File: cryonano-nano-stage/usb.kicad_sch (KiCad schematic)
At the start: 5 parts, among them J4 10118194-0001LF, U10 ECMF02-2AMX6

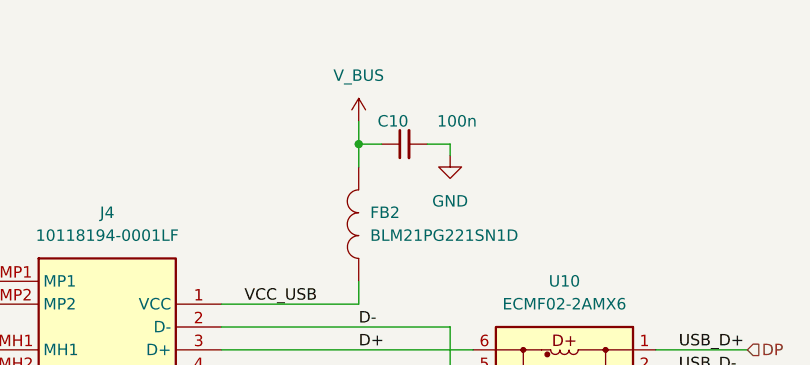
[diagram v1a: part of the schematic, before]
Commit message: partially populated
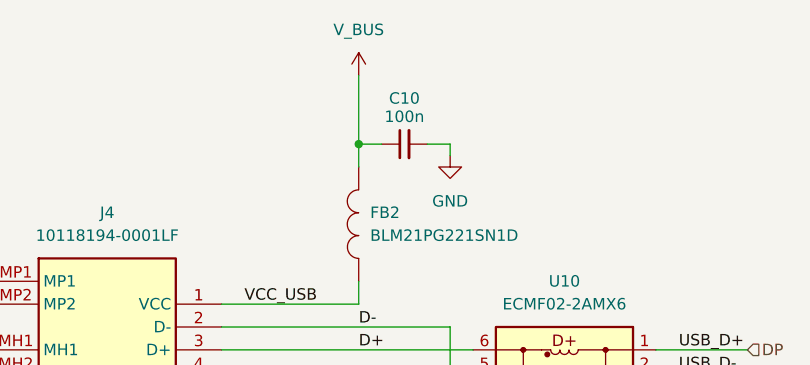
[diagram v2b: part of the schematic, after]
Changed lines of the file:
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@@
+	)
+	(junction
+		(at 60.96 66.04)
+		(diameter 0)
+		(color 0 0 0 0)
 	)
 	(junction
@@
 	)
 	(junction
-		(at 60.96 66.04)
-		(diameter 0)
-		(color 0 0 0 0)
-	)
-	(junction
 		(at 60.96 76.2)
 		(diameter 0)
@@
 	(wire
 		(pts
-			(xy 104.14 48.26) (xy 104.14 45.72)
+			(xy 104.14 48.26) (xy 104.14 40.64)
 		)
 		(stroke
@@
 	(symbol
 		(lib_id "interface-pcb:V_BUS")
-		(at 104.14 45.72 0)
+		(at 104.14 40.64 0)
 		(unit 1)
 		(body_style 1)
@@
 		(fields_autoplaced yes)
 		(property "Reference" "#PWR0242"
-			(at 104.14 49.53 0)
+			(at 104.14 44.45 0)
 			(hide yes)
 			(show_name no)
@@
 		)
 		(property "Value" "V_BUS"
+			(at 104.14 35.56 0)
+			(show_name no)
+			(do_not_autoplace no)
+			(effects
+				(font
+					(size 1.27 1.27)
+				)
+			)
+		)
+		(property "Footprint" ""
 			(at 104.14 40.64 0)
-			(show_name no)
-			(do_not_autoplace no)
-			(effects
-				(font
-					(size 1.27 1.27)
-				)
-			)
-		)
-		(property "Footprint" ""
-			(at 104.14 45.72 0)
 			(hide yes)
 			(show_name no)
@@
 		)
 		(property "Datasheet" ""
-			(at 104.14 45.72 0)
+			(at 104.14 40.64 0)
 			(hide yes)
 			(show_name no)
@@
 		)
 		(property "Description" ""
-			(at 104.14 45.72 0)
+			(at 104.14 40.64 0)
 			(hide yes)
 			(show_name no)
@@
 		(dnp no)
 		(property "Reference" "C10"
-			(at 107.95 45.72 90)
+			(at 109.22 43.18 90)
 			(show_name no)
 			(do_not_autoplace no)
@@
 		)
 		(property "Value" "100n"
-			(at 115.062 45.72 90)
-			(show_name no)
-			(do_not_autoplace no)
+			(at 109.22 45.212 90)
+			(show_name no)
+			(do_not_autoplace no)

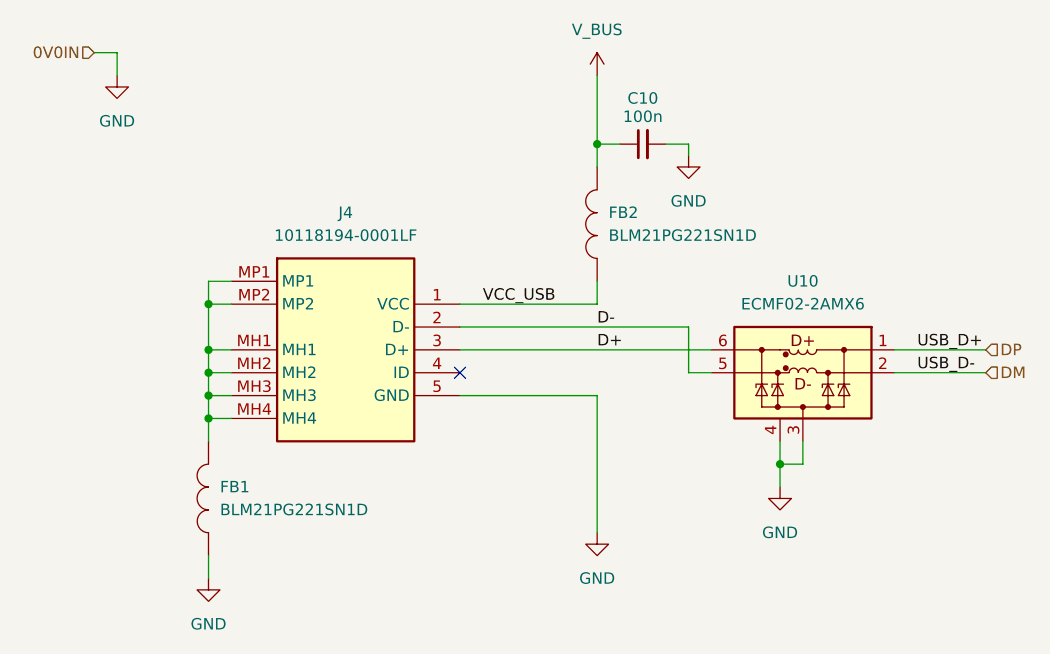
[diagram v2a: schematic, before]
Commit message: sch improved
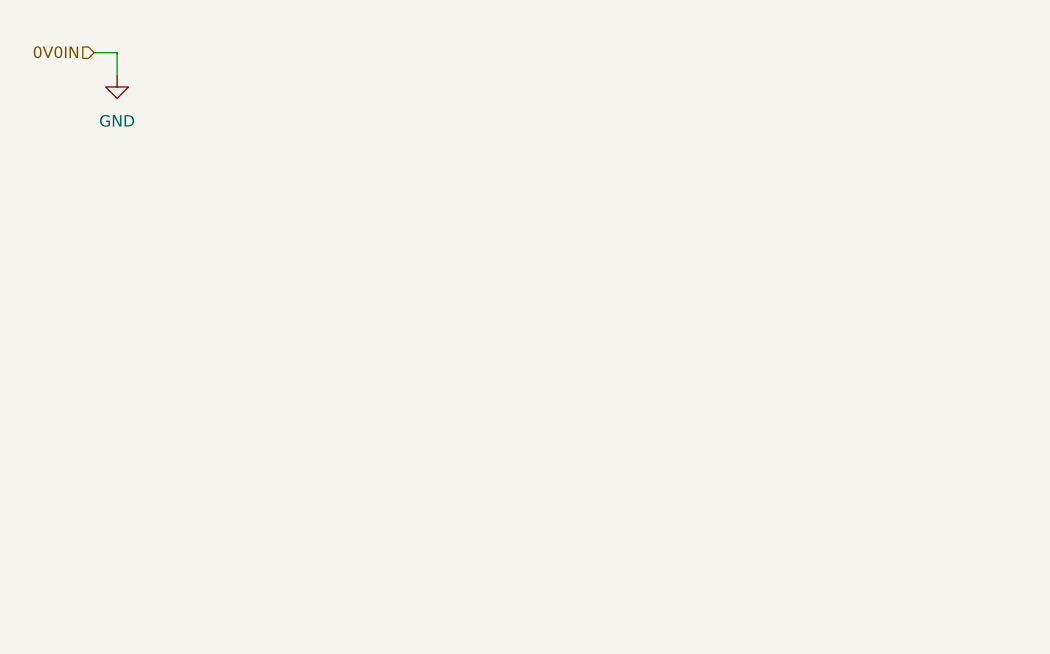
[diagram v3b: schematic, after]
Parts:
- removed C10: 100n, Capacitor_SMD:C_0603_1608Metric, symbol interface-pcb:C_Small
- removed FB1, FB2: BLM21PG221SN1D, Inductor_SMD:L_0805_2012Metric, symbol symbols:BLM21PG221SN1D
- removed J4: 10118194-0001LF, footprints:101181940001LF, symbol symbols:10118194-0001LF
- removed U10: ECMF02-2AMX6, Package_DFN_QFN:ST_UQFN-6L_1.5x1.7mm_P0.5mm, symbol symbols:ECMF02-2AMX6
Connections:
- no-connect marks 1 -> 0
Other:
- company: (none) -> Cryonano Labs Pvt. Ltd.
- title: (none) -> Nano stage controller
